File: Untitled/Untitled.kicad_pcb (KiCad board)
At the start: 2 copper layers, 114 x 78 mm, 3 parts, among them J1 Screw_Terminal_01x04, J2 Screw_Terminal_01x04, U1 Pico

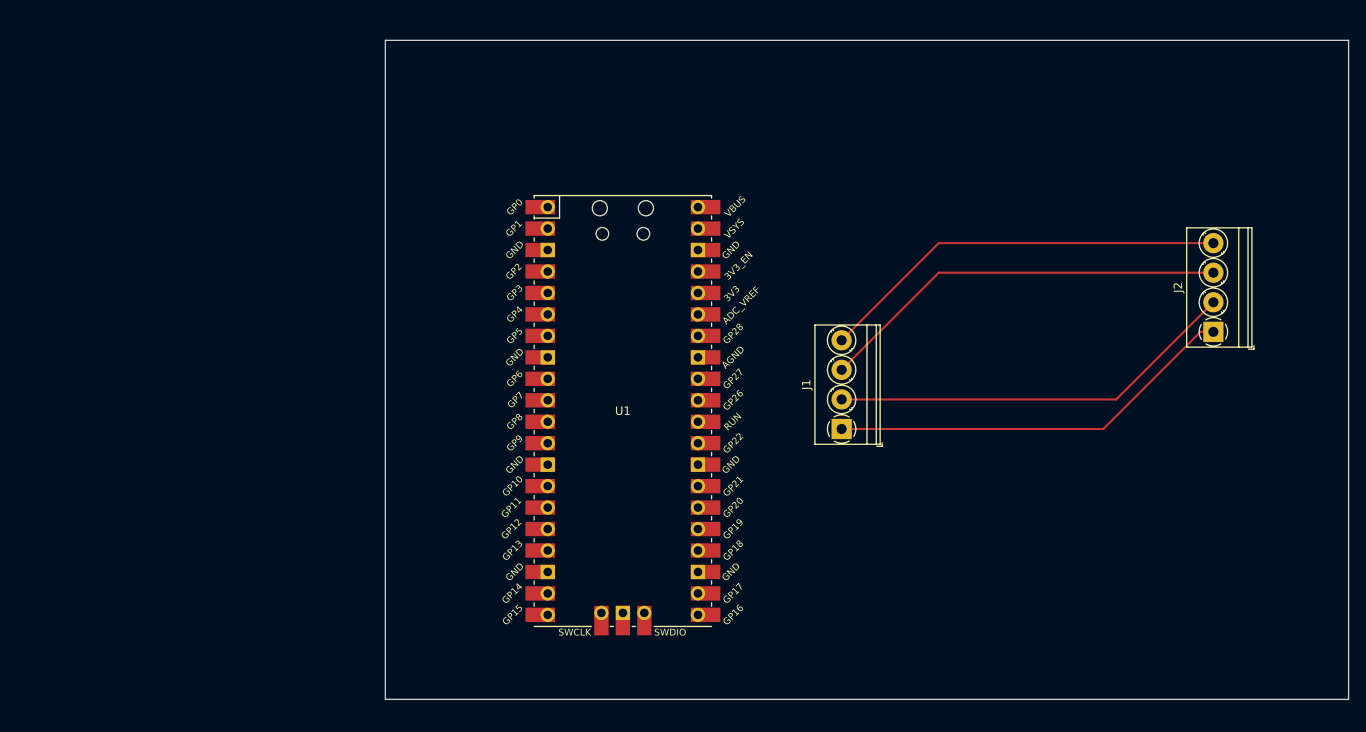
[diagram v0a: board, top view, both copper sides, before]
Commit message: 08/09/25 20:07 Titan.local
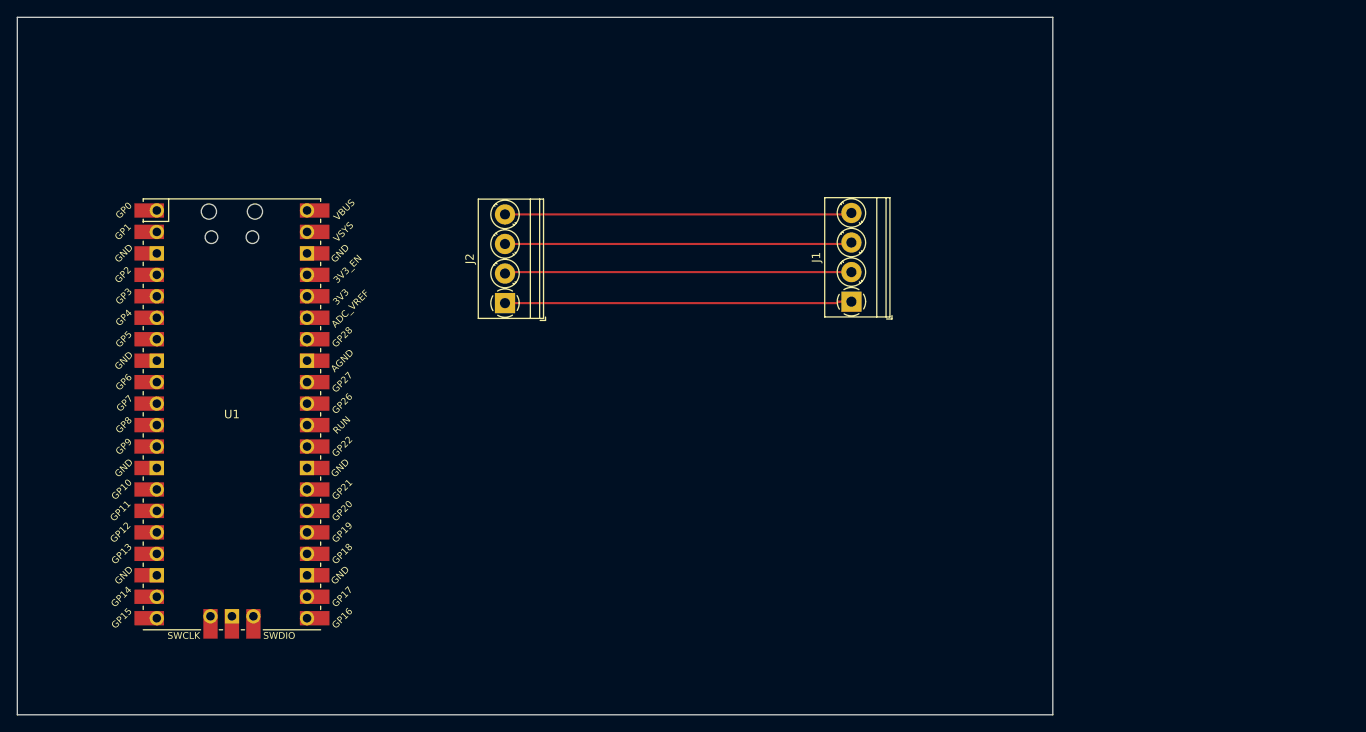
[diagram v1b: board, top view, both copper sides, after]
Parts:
- moved J2 83.9 mm to (149.2, 75.1)
- moved U1 46.3 mm to (116.8, 88.3)
- moved J1 15.1 mm to (190.2, 74.9)
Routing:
- net Net-(J1-Pin_2): track 48.8 -> 41.1 mm
- net Net-(J1-Pin_1): track 48.8 -> 41.1 mm
- net Net-(J1-Pin_4): track 48.8 -> 41.1 mm
- net Net-(J1-Pin_3): track 48.8 -> 41.1 mm
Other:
- board size 114 x 78 mm -> 122.6 x 82.6 mm
